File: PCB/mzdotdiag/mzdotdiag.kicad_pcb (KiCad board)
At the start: 2 copper layers, 45 parts, among them J1 Conn_01x25, J2 RST, J3 BOOT, J4 UART, Q10 Q_NPN_BEC, Q11 Q_NPN_BEC, Q17 Q_NPN_BEC, Q9 Q_NPN_BEC, SW1 SW_Push, U3 ESP32-WROOM-32, U4 MC14504B, U5 MC14504B

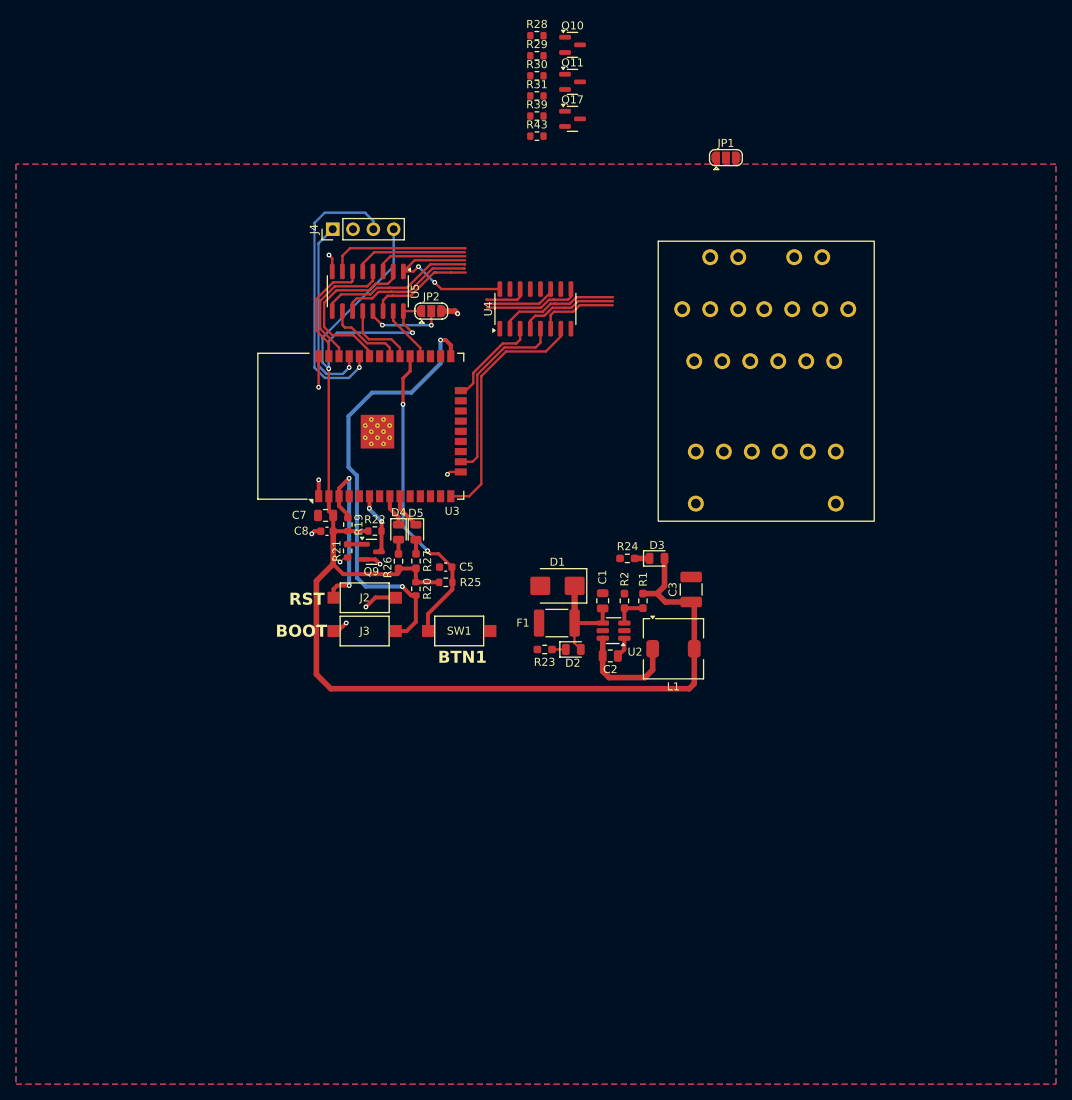
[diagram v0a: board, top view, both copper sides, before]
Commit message: finished wiring
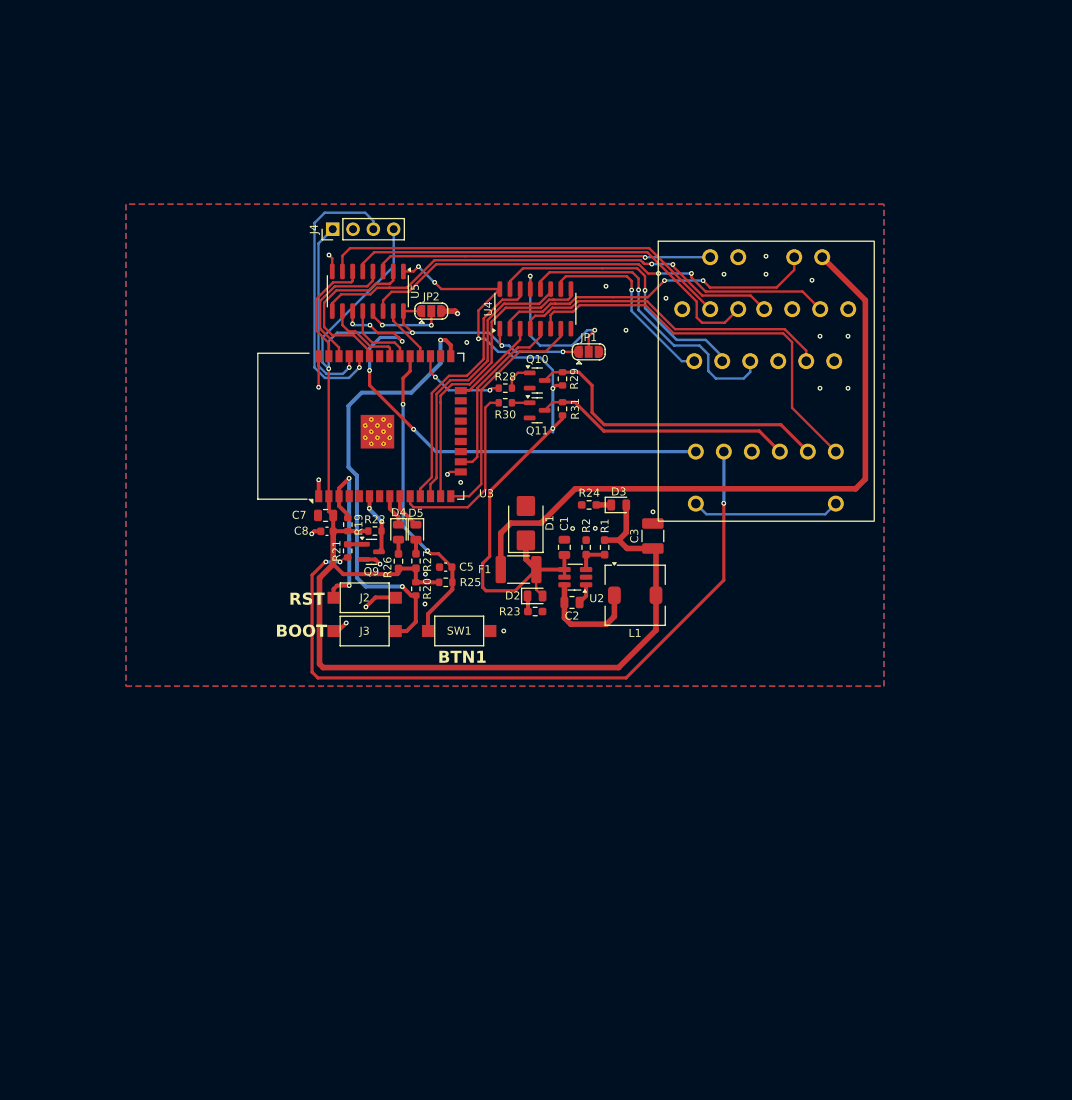
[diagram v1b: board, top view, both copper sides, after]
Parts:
- removed Q17: Q_NPN_BEC, Package_TO_SOT_SMD:SOT-23
- removed R39: 1k, Resistor_SMD:R_0603_1608Metric
- removed R43: 10k, Resistor_SMD:R_0603_1608Metric
- moved R28 44.2 mm to (111.2, 68.0)
- moved Q10 42.2 mm to (115.2, 67.0)
- moved Q11 41.3 mm to (115.1, 70.8)
- moved R30 41.1 mm to (111.2, 69.8)
- moved R29 40.5 mm to (118.3, 66.8), turned to 90 degrees
- moved R31 39.2 mm to (118.3, 70.6), turned to 90 degrees
- moved JP1 29.7 mm to (121.6, 63.5)
- moved D1 8.77 mm to (113.7, 84.9), turned to 90 degrees
- moved D2 8.22 mm to (114.9, 94.0)
- moved F1 8.22 mm to (112.8, 90.7)
- moved R1 8.22 mm to (123.6, 87.9)
- moved R2 8.22 mm to (121.3, 87.9)
- moved C1 8.22 mm to (118.5, 87.9)
- moved C2 8.22 mm to (119.5, 94.8)
- moved C3 8.22 mm to (129.6, 86.5)
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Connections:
- C1 pad 2: Net-(D1-K) -> /B+_PROT
- D1 pad 1: Net-(D1-K) -> /B+_PROT
- D2 pad 2: Net-(D1-K) -> /B+_PROT
- F1 pad 2: Net-(D1-K) -> /B+_PROT
- R29 pad 1: /B+ -> /B+_PROT
- R31 pad 1: /B+ -> /B+_PROT
- U2 pad 4: Net-(D1-K) -> /B+_PROT
- U2 pad 5: Net-(D1-K) -> /B+_PROT
- U3 pad 10: unconnected-(U3-IO25-Pad10) -> /ESP32_TFA
- U3 pad 11: unconnected-(U3-IO26-Pad11) -> /ESP32_TBS
- U3 pad 12: unconnected-(U3-IO27-Pad12) -> /ESP32_TAC
- U4 pad 16: /B+ -> /B+_PROT
- U5 pad 1: /B+ -> /B+_PROT
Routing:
- net /IG-: track 1.19 -> 90.5 mm, vias 1 -> 3
- net /B+_PROT: track 0.00 -> 88.6 mm, vias 0 -> 5
- net /B+: track 21.8 -> 82.9 mm, vias 2 -> 0
- net /FSC: track 13.1 -> 60.5 mm, vias 0 -> 2
- net /FAB: track 16.9 -> 62.4 mm, vias 0 -> 5
- net /FAC: track 19.6 -> 59.9 mm, vias 0 -> 2
- net /TAB: track 9.97 -> 50.2 mm
- net /FBS: track 14.4 -> 54.0 mm
- net /F/P: track 0.00 -> 39.4 mm
- net /TAC: track 0.00 -> 38.4 mm, vias 0 -> 1
- net /TBS: track 0.00 -> 35.7 mm, vias 0 -> 1
- net /FAT: track 17.7 -> 51.5 mm
- net /TFA: track 0.00 -> 32.4 mm
- net /FEN: track 11.6 -> 42.3 mm, vias 0 -> 1
- net /ESP32_TBS: track 5.34 -> 33.5 mm
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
